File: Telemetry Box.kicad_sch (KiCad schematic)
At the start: 2 parts

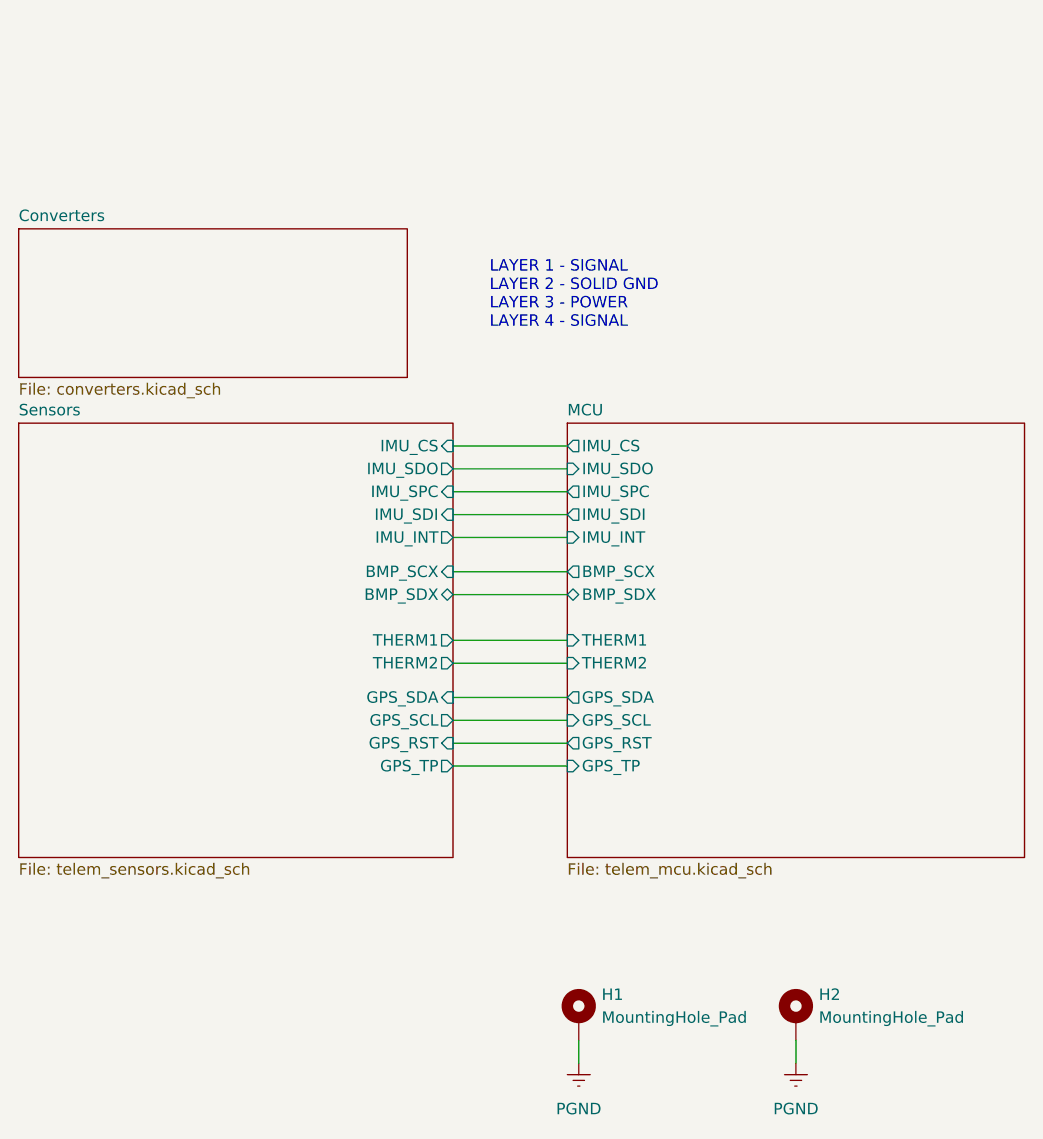
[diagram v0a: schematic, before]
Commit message: Updated schematics for rev2
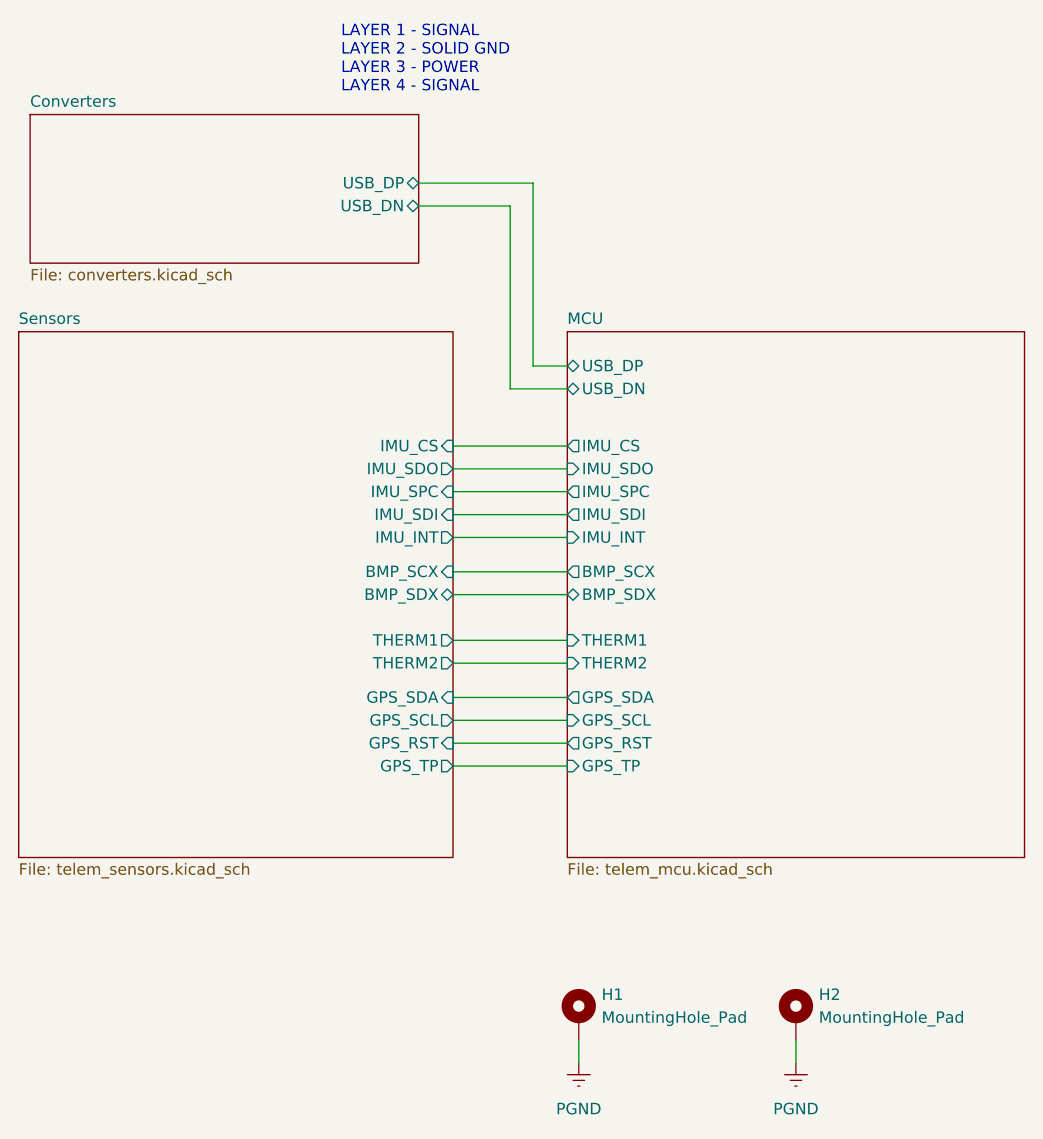
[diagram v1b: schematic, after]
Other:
- sheet Converters ports: added USB_DN, USB_DP; removed none
- sheet MCU ports: added USB_DN, USB_DP; removed none
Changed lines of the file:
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@@
 	(text "LAYER 1 - SIGNAL\nLAYER 2 - SOLID GND\nLAYER 3 - POWER\nLAYER 4 - SIGNAL"
 		(exclude_from_sim no)
-		(at 94.234 72.136 0)
+		(at 77.724 45.974 0)
 		(effects
 			(font
@@
 	(wire
 		(pts
+			(xy 90.17 119.38) (xy 102.87 119.38)
+		)
+		(stroke
+			(width 0)
+			(type default)
+		)
+	)
+	(wire
+		(pts
+			(xy 90.17 110.49) (xy 102.87 110.49)
+		)
+		(stroke
+			(width 0)
+			(type default)
+		)
+	)
+	(wire
+		(pts
+			(xy 104.14 154.94) (xy 104.14 157.48)
+		)
+		(stroke
+			(width 0)
+			(type default)
+		)
+	)
+	(wire
+		(pts
 			(xy 90.17 124.46) (xy 102.87 124.46)
 		)
@@
 	(wire
 		(pts
-			(xy 90.17 119.38) (xy 102.87 119.38)
-		)
-		(stroke
-			(width 0)
-			(type default)
-		)
-	)
-	(wire
-		(pts
-			(xy 90.17 110.49) (xy 102.87 110.49)
-		)
-		(stroke
-			(width 0)
-			(type default)
-		)
-	)
-	(wire
-		(pts
-			(xy 104.14 154.94) (xy 104.14 157.48)
+			(xy 96.52 82.55) (xy 102.87 82.55)
 		)
 		(stroke
@@
 	(wire
 		(pts
+			(xy 86.36 59.69) (xy 99.06 59.69)
+		)
+		(stroke
+			(width 0)
+			(type default)
+		)
+	)
+	(wire
+		(pts
 			(xy 90.17 113.03) (xy 102.87 113.03)
 		)
@@
 	(wire
 		(pts
+			(xy 99.06 59.69) (xy 99.06 80.01)
+		)
+		(stroke
+			(width 0)
+			(type default)
+		)
+	)
+	(wire
+		(pts
+			(xy 99.06 80.01) (xy 102.87 80.01)
+		)
+		(stroke
+			(width 0)
+			(type default)
+		)
+	)
+	(wire
+		(pts
 			(xy 90.17 96.52) (xy 102.87 96.52)
 		)
@@
 	(wire
 		(pts
+			(xy 86.36 62.23) (xy 96.52 62.23)
+		)
+		(stroke
+			(width 0)
+			(type default)
+		)
+	)
+	(wire
+		(pts
 			(xy 90.17 88.9) (xy 102.87 88.9)
 		)
@@
 		(pts
 			(xy 90.17 121.92) (xy 102.87 121.92)
+		)
+		(stroke
+			(width 0)
+			(type default)
+		)
+	)
+	(wire
+		(pts
+			(xy 96.52 62.23) (xy 96.52 82.55)
 		)
 		(stroke
@@
 	)
 	(sheet
-		(at 41.91 86.36)
-		(size 48.26 48.26)
+		(at 41.91 76.2)
+		(size 48.26 58.42)
 		(exclude_from_sim no)
 		(in_bom yes)
@@
 		)
 		(property "Sheetname" "Sensors"
-			(at 41.91 85.6484 0)
+			(at 41.91 75.4884 0)
 			(show_name no)
 			(do_not_autoplace no)
@@
 		)
 		(property "Field2" ""
-			(at 41.91 86.36 0)
+			(at 41.91 76.2 0)
 			(hide yes)
 			(show_name no)
@@
 	)
 	(sheet
-		(at 102.87 86.36)
-		(size 50.8 48.26)
+		(at 102.87 76.2)
+		(size 50.8 58.42)
 		(exclude_from_sim no)
 		(in_bom yes)
@@
 		)
 		(property "Sheetname" "MCU"
-			(at 102.87 85.6484 0)
+			(at 102.87 75.4884 0)
 			(show_name no)
 			(do_not_autoplace no)
@@
 		(pin "GPS_SCL" input
 			(at 102.87 119.38 180)
+			(effects
+				(font
+					(size 1.27 1.27)
+				)
+				(justify left)
+			)
+		)
+		(pin "USB_DN" bidirectional
+			(at 102.87 82.55 180)
+			(effects
+				(font
+					(size 1.27 1.27)
+				)
+				(justify left)
+			)
+		)
+		(pin "USB_DP" bidirectional
+			(at 102.87 80.01 180)
 			(effects
 				(font
@@
 	)
 	(sheet
-		(at 41.91 64.77)
+		(at 43.18 52.07)
 		(size 43.18 16.51)
 		(exclude_from_sim no)
@@
 		)
 		(property "Sheetname" "Converters"
-			(at 41.91 64.0584 0)
+			(at 43.18 51.3584 0)
 			(show_name no)
 			(do_not_autoplace no)
@@
 		)
 		(property "Sheetfile" "converters.kicad_sch"
-			(at 41.91 81.8646 0)
+			(at 43.18 69.1646 0)
 			(show_name no)
 			(do_not_autoplace no)
@@
 		)
 		(property "Field2" ""
-			(at 41.91 64.77 0)
-			(hide yes)
-			(show_name no)
-			(do_not_autoplace no)
-			(effects
-				(font
-					(size 1.27 1.27)
-				)
-			)
-		)
+			(at 43.18 52.07 0)
+			(hide yes)
+			(show_name no)
+			(do_not_autoplace no)
+			(effects
+				(font
+					(size 1.27 1.27)
+				)
+			)
+		)
+		(pin "USB_DN" bidirectional
+			(at 86.36 62.23 0)
+			(effects
+				(font
+					(size 1.27 1.27)
+				)
+				(justify right)
+			)
+		)
+		(pin "USB_DP" bidirectional
+			(at 86.36 59.69 0)
+			(effects
+				(font
+					(size 1.27 1.27)
+				)
+				(justify right)
+			)
+		)
